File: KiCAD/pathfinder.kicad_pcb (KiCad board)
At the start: 2 copper layers, 66.2 x 42.5 mm, 10 parts, among them SW1 SW_Push, SW2 SW_Push, SW3 SW_Push, U1 MOUDLE-SEEEDUINO-XIAO

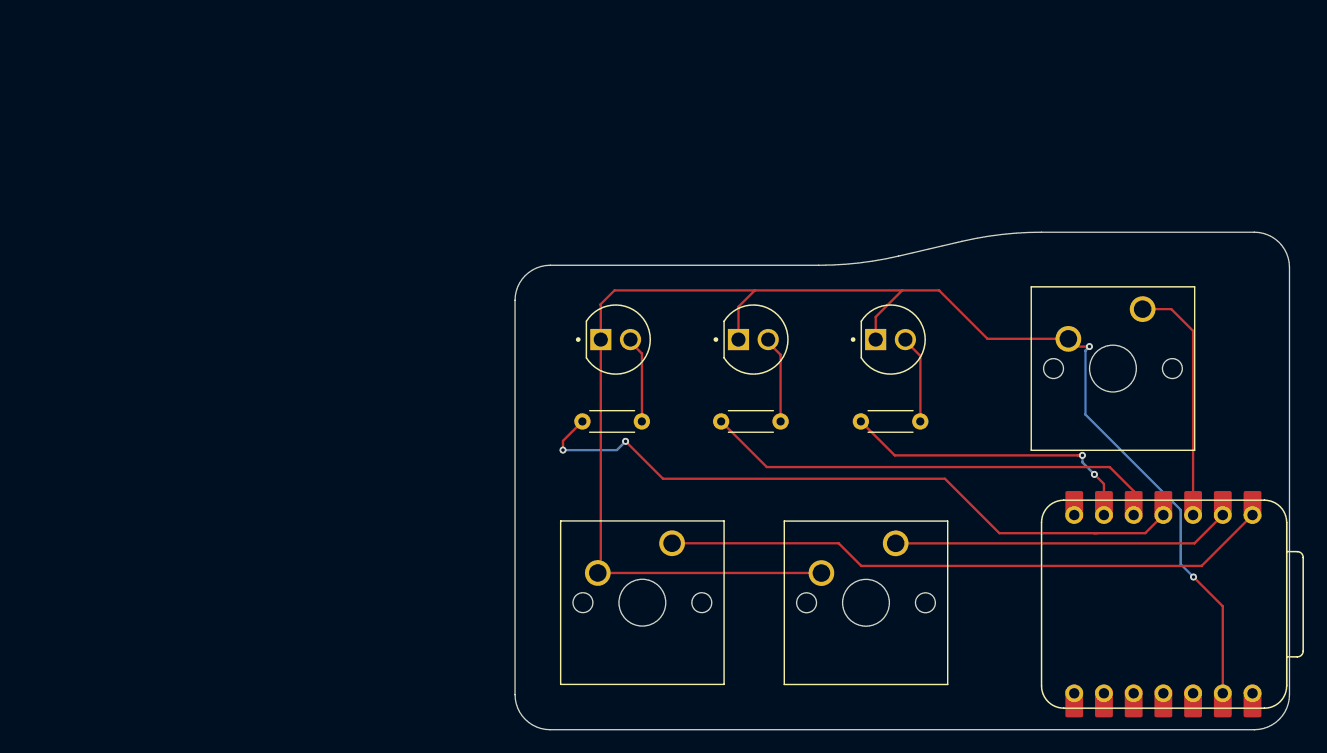
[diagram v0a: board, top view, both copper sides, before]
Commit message: pcb making + firmware
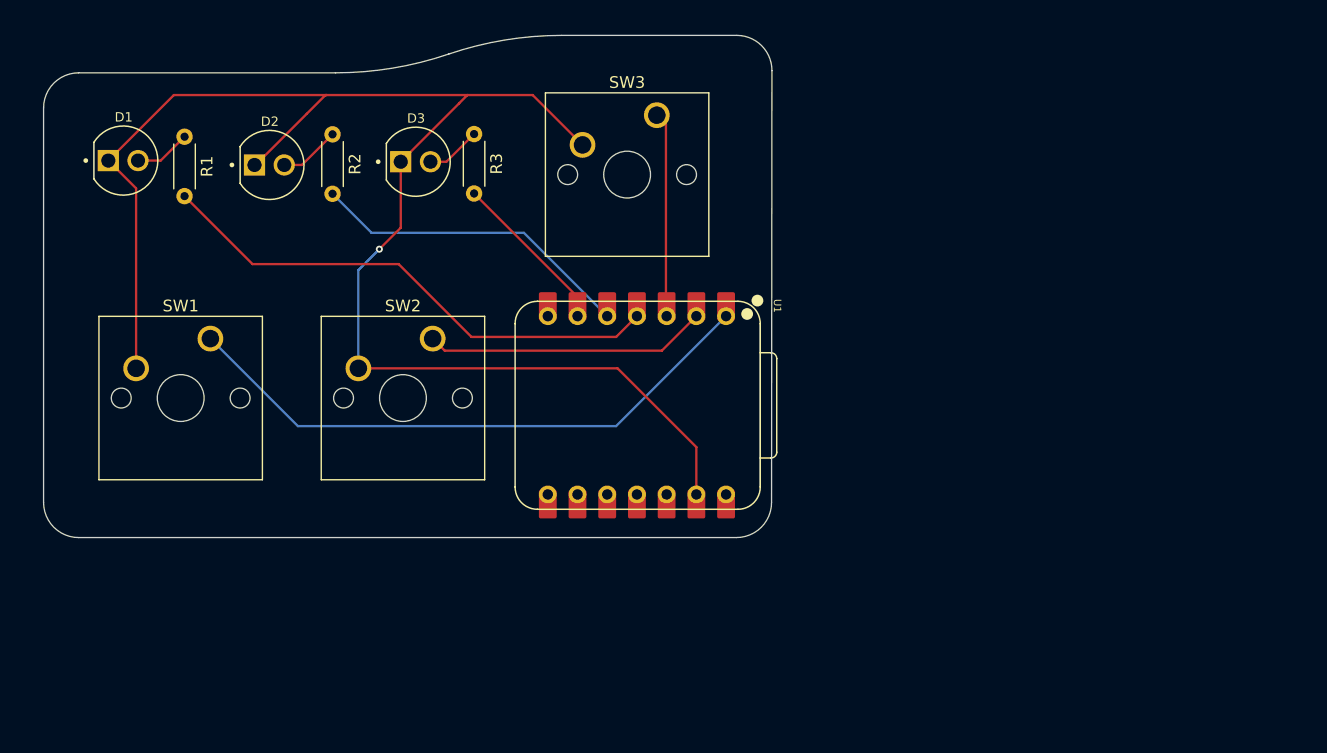
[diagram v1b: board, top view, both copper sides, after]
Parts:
- removed D4, D5, D6: L08R5000Q1, footprints:LEDRD254W57D500H1070
- added D1: L08R5000Q1, footprints:LEDRD254W57D500H1070, F.Cu at (121.0, 52.7)
- added D2: L08R5000Q1, footprints:LEDRD254W57D500H1070, F.Cu at (133.5, 53.1)
- added D3: L08R5000Q1, footprints:LEDRD254W57D500H1070, F.Cu at (146.0, 52.8)
- U1: value MOUDLE-SEEEDUINO-XIAO -> XIAO-RP2040-DIP; footprint megapad:XIAO-RP2040-DIP -> footprints:XIAO-RP2040-DIP
- moved U1 48.1 mm to (164.9, 73.6)
- moved R1 46.0 mm to (126.2, 50.7), turned to -90 degrees
- moved R2 45.5 mm to (138.9, 50.5), turned to -90 degrees
- moved R3 45.4 mm to (151.0, 50.4), turned to -90 degrees
- moved SW3 44.7 mm to (166.6, 48.8)
- moved SW2 43.3 mm to (147.5, 67.9)
- moved SW1 43.2 mm to (128.5, 67.9)
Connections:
- net GPIO0 renamed button1
- net GPIO1 renamed button2
- net GPIO2 renamed button3
- net GPIO3 renamed LED1
- net GPIO4 renamed LED2
- net GPIO5 renamed LED3
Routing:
- net LED1: track 59.0 -> 44.4 mm, vias 2 -> 0
- net LED2: track 39.8 -> 27.8 mm
- net LED3: track 25.2 -> 13.3 mm, vias 2 -> 0
- net button2: track 29.0 -> 24.2 mm
- net button3: track 20.8 -> 16.7 mm
- net GND: track 131.0 -> 134.9 mm, vias 2 -> 1
- net Net-(D1-PadA): track 7.66 -> 4.82 mm
- net Net-(D3-PadA): track 7.22 -> 4.71 mm
- net Net-(D2-PadA): track 7.22 -> 5.21 mm
- net button1: track 52.2 -> 51.1 mm
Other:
- board size 66.2 x 42.5 mm -> 62.3 x 42.9 mm

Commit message: code formatting
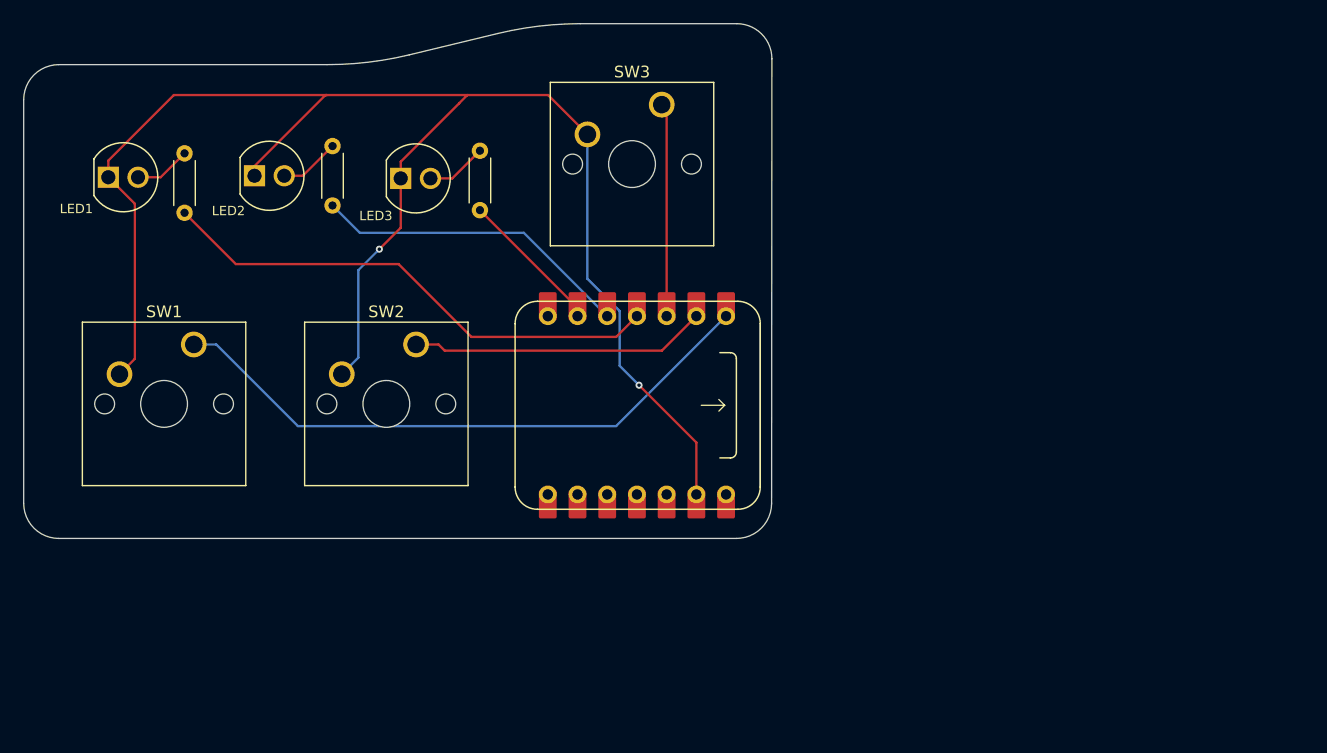
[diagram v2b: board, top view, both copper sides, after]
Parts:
- moved R3 1.51 mm to (151.5, 51.9)
- moved SW2 1.51 mm to (146.0, 68.4)
- moved SW1 1.51 mm to (127.0, 68.4)
- moved LED3 1.43 mm to (146.0, 54.2)
- moved R1 1.43 mm to (126.2, 52.1)
- moved LED1 1.42 mm to (121.0, 54.1)
- moved R2 1.00 mm to (138.9, 51.5)
- moved SW3 0.99 mm to (167.0, 47.9)
- moved LED2 0.92 mm to (133.5, 54.0)
- renumbered D1 to LED1, D2 to LED2, D3 to LED3
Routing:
- net GND: track 134.9 -> 136.9 mm, vias 1 -> 2
- net button2: track 24.2 -> 25.4 mm
- net button1: track 51.1 -> 52.3 mm
- net button3: track 16.7 -> 17.5 mm
- net LED3: track 13.3 -> 12.6 mm
- net LED1: track 44.4 -> 43.8 mm
- net Net-(D3-PadA): track 4.71 -> 5.21 mm
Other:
- board size 62.3 x 42.9 mm -> 64 x 44 mm
